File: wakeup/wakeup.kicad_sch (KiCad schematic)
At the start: 15 parts, among them J1 Conn_01x03_Female, U1 74HC00, U2 74HC393

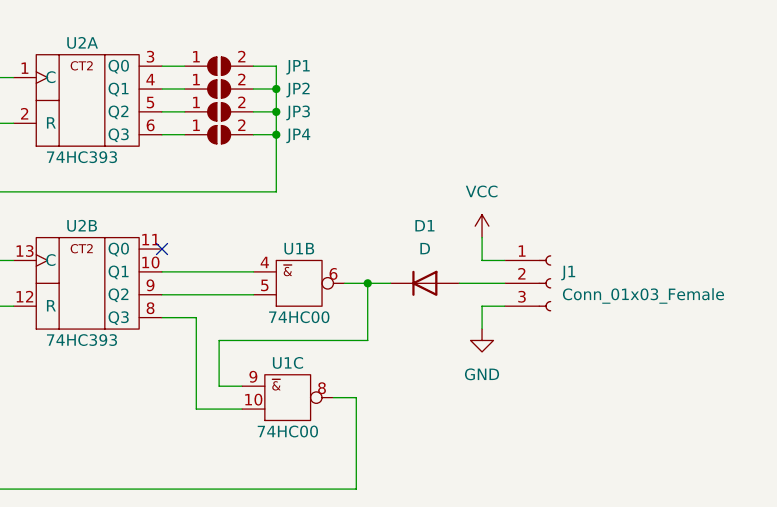
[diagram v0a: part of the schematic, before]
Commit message: non function changes
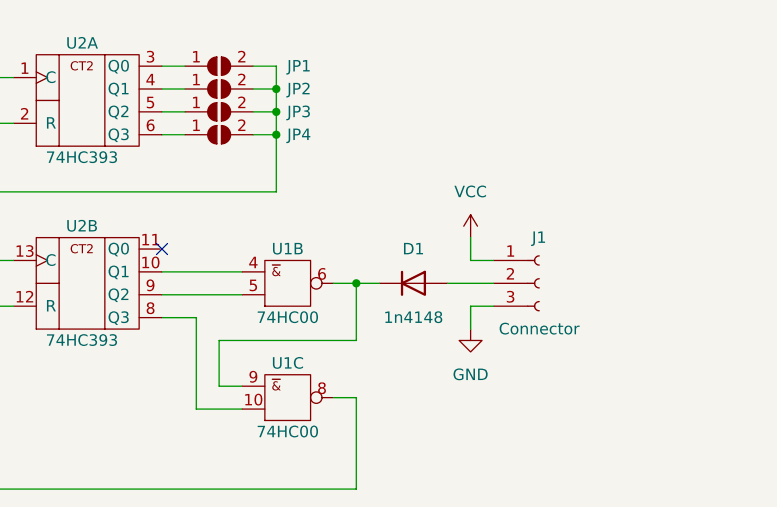
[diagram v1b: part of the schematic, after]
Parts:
- D1: value D -> 1n4148
- J1: value Conn_01x03_Female -> Connector
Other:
- moved on the sheet: D1, J1, U1B
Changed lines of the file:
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@@
   (junction (at 135.89 68.58) (diameter 0) (color 0 0 0 0)
   )
-  (junction (at 146.05 87.63) (diameter 0) (color 0 0 0 0)
+  (junction (at 144.78 87.63) (diameter 0) (color 0 0 0 0)
   )
   (junction (at 101.6 90.17) (diameter 0) (color 0 0 0 0)
@@
     (stroke (width 0) (type default) (color 0 0 0 0))
   )
-  (wire (pts (xy 158.75 92.71) (xy 158.75 90.17))
+  (wire (pts (xy 157.48 92.71) (xy 157.48 90.17))
     (stroke (width 0) (type default) (color 0 0 0 0))
   )
@@
     (stroke (width 0) (type default) (color 0 0 0 0))
   )
-  (wire (pts (xy 146.05 87.63) (xy 148.59 87.63))
+  (wire (pts (xy 144.78 87.63) (xy 147.32 87.63))
     (stroke (width 0) (type default) (color 0 0 0 0))
   )
@@
     (stroke (width 0) (type default) (color 0 0 0 0))
   )
-  (wire (pts (xy 158.75 82.55) (xy 158.75 85.09))
+  (wire (pts (xy 157.48 82.55) (xy 157.48 85.09))
     (stroke (width 0) (type default) (color 0 0 0 0))
   )
@@
     (stroke (width 0) (type default) (color 0 0 0 0))
   )
-  (wire (pts (xy 158.75 85.09) (xy 161.29 85.09))
+  (wire (pts (xy 157.48 85.09) (xy 160.02 85.09))
     (stroke (width 0) (type default) (color 0 0 0 0))
   )
@@
     (stroke (width 0) (type default) (color 0 0 0 0))
   )
-  (wire (pts (xy 146.05 93.98) (xy 129.54 93.98))
+  (wire (pts (xy 144.78 93.98) (xy 129.54 93.98))
     (stroke (width 0) (type default) (color 0 0 0 0))
   )
@@
     (stroke (width 0) (type default) (color 0 0 0 0))
   )
-  (wire (pts (xy 156.21 87.63) (xy 161.29 87.63))
+  (wire (pts (xy 154.94 87.63) (xy 160.02 87.63))
     (stroke (width 0) (type default) (color 0 0 0 0))
   )
@@
     (stroke (width 0) (type default) (color 0 0 0 0))
   )
-  (wire (pts (xy 146.05 87.63) (xy 146.05 93.98))
+  (wire (pts (xy 144.78 87.63) (xy 144.78 93.98))
     (stroke (width 0) (type default) (color 0 0 0 0))
   )
@@
     (stroke (width 0) (type default) (color 0 0 0 0))
   )
-  (wire (pts (xy 143.51 87.63) (xy 146.05 87.63))
+  (wire (pts (xy 142.24 87.63) (xy 144.78 87.63))
     (stroke (width 0) (type default) (color 0 0 0 0))
   )
@@
     (stroke (width 0) (type default) (color 0 0 0 0))
   )
-  (wire (pts (xy 158.75 90.17) (xy 161.29 90.17))
+  (wire (pts (xy 157.48 90.17) (xy 160.02 90.17))
     (stroke (width 0) (type default) (color 0 0 0 0))
   )
@@
     (stroke (width 0) (type default) (color 0 0 0 0))
   )
-  (wire (pts (xy 123.19 88.9) (xy 133.35 88.9))
+  (wire (pts (xy 123.19 88.9) (xy 132.08 88.9))
     (stroke (width 0) (type default) (color 0 0 0 0))
   )
@@
     (stroke (width 0) (type default) (color 0 0 0 0))
   )
-  (wire (pts (xy 123.19 86.36) (xy 133.35 86.36))
+  (wire (pts (xy 123.19 86.36) (xy 132.08 86.36))
     (stroke (width 0) (type default) (color 0 0 0 0))
   )
@@
     (pin "2")
   )
-  (symbol (lib_id "power:GND") (at 158.75 92.71 0) (unit 1)
-    (in_bom yes) (on_board yes) (fields_autoplaced)
-    (property "Reference" "#PWR07" (id 0) (at 158.75 99.06 0)
-      (effects (font (size 1.27 1.27)) hide)
-    )
-    (property "Value" "GND" (id 1) (at 158.75 97.79 0))
-    (property "Footprint" "" (id 2) (at 158.75 92.71 0)
-      (effects (font (size 1.27 1.27)) hide)
-    )
-    (property "Datasheet" "" (id 3) (at 158.75 92.71 0)
+  (symbol (lib_id "power:GND") (at 157.48 92.71 0) (unit 1)
+    (in_bom yes) (on_board yes) (fields_autoplaced)
+    (property "Reference" "#PWR07" (id 0) (at 157.48 99.06 0)
+      (effects (font (size 1.27 1.27)) hide)
+    )
+    (property "Value" "GND" (id 1) (at 157.48 97.79 0))
+    (property "Footprint" "" (id 2) (at 157.48 92.71 0)
+      (effects (font (size 1.27 1.27)) hide)
+    )
+    (property "Datasheet" "" (id 3) (at 157.48 92.71 0)
       (effects (font (size 1.27 1.27)) hide)
     )
@@
     (pin "13")
   )
-  (symbol (lib_id "74IEC:74HC00") (at 138.43 87.63 0) (unit 2)
-    (in_bom yes) (on_board yes)
-    (property "Reference" "U1" (id 0) (at 138.43 83.82 0))
-    (property "Value" "74HC00" (id 1) (at 138.43 91.44 0))
-    (property "Footprint" "Package_SO:SO-14_3.9x8.65mm_P1.27mm" (id 2) (at 138.43 93.98 0)
-      (effects (font (size 1.27 1.27)) hide)
-    )
-    (property "Datasheet" "https://www.ti.com/lit/ds/symlink/sn7400.pdf" (id 3) (at 138.43 83.82 0)
+  (symbol (lib_id "74IEC:74HC00") (at 137.16 87.63 0) (unit 2)
+    (in_bom yes) (on_board yes)
+    (property "Reference" "U1" (id 0) (at 137.16 83.82 0))
+    (property "Value" "74HC00" (id 1) (at 137.16 91.44 0))
+    (property "Footprint" "Package_SO:SO-14_3.9x8.65mm_P1.27mm" (id 2) (at 137.16 93.98 0)
+      (effects (font (size 1.27 1.27)) hide)
+    )
+    (property "Datasheet" "https://www.ti.com/lit/ds/symlink/sn7400.pdf" (id 3) (at 137.16 83.82 0)
       (effects (font (size 1.27 1.27)) hide)
     )
@@
     (pin "2")
   )
-  (symbol (lib_id "Device:D") (at 152.4 87.63 0) (unit 1)
-    (in_bom yes) (on_board yes) (fields_autoplaced)
-    (property "Reference" "D1" (id 0) (at 152.4 81.28 0))
-    (property "Value" "D" (id 1) (at 152.4 83.82 0))
-    (property "Footprint" "" (id 2) (at 152.4 87.63 0)
-      (effects (font (size 1.27 1.27)) hide)
-    )
-    (property "Datasheet" "~" (id 3) (at 152.4 87.63 0)
+  (symbol (lib_id "Device:D") (at 151.13 87.63 0) (unit 1)
+    (in_bom yes) (on_board yes)
+    (property "Reference" "D1" (id 0) (at 151.13 83.82 0))
+    (property "Value" "1n4148" (id 1) (at 151.13 91.44 0))
+    (property "Footprint" "" (id 2) (at 151.13 87.63 0)
+      (effects (font (size 1.27 1.27)) hide)
+    )
+    (property "Datasheet" "~" (id 3) (at 151.13 87.63 0)
       (effects (font (size 1.27 1.27)) hide)
     )
@@
     (pin "9")
   )
-  (symbol (lib_id "power:VCC") (at 158.75 82.55 0) (unit 1)
-    (in_bom yes) (on_board yes) (fields_autoplaced)
-    (property "Reference" "#PWR05" (id 0) (at 158.75 86.36 0)
-      (effects (font (size 1.27 1.27)) hide)
-    )
-    (property "Value" "VCC" (id 1) (at 158.75 77.47 0))
-    (property "Footprint" "" (id 2) (at 158.75 82.55 0)
-      (effects (font (size 1.27 1.27)) hide)
-    )
-    (property "Datasheet" "" (id 3) (at 158.75 82.55 0)
+  (symbol (lib_id "power:VCC") (at 157.48 82.55 0) (unit 1)
+    (in_bom yes) (on_board yes) (fields_autoplaced)
+    (property "Reference" "#PWR05" (id 0) (at 157.48 86.36 0)
+      (effects (font (size 1.27 1.27)) hide)
+    )
+    (property "Value" "VCC" (id 1) (at 157.48 77.47 0))
+    (property "Footprint" "" (id 2) (at 157.48 82.55 0)
+      (effects (font (size 1.27 1.27)) hide)
+    )
+    (property "Datasheet" "" (id 3) (at 157.48 82.55 0)
       (effects (font (size 1.27 1.27)) hide)
     )
@@
     (pin "13")
   )
-  (symbol (lib_id "Connector:Conn_01x03_Female") (at 166.37 87.63 0) (unit 1)
-    (in_bom yes) (on_board yes) (fields_autoplaced)
-    (property "Reference" "J1" (id 0) (at 167.64 86.3599 0)
-      (effects (font (size 1.27 1.27)) (justify left))
-    )
-    (property "Value" "Conn_01x03_Female" (id 1) (at 167.64 88.8999 0)
-      (effects (font (size 1.27 1.27)) (justify left))
-    )
-    (property "Footprint" "Connector_PinSocket_2.54mm:PinSocket_1x03_P2.54mm_Vertical" (id 2) (at 166.37 87.63 0)
-      (effects (font (size 1.27 1.27)) hide)
-    )
-    (property "Datasheet" "~" (id 3) (at 166.37 87.63 0)
+  (symbol (lib_id "Connector:Conn_01x03_Female") (at 165.1 87.63 0) (unit 1)
+    (in_bom yes) (on_board yes)
+    (property "Reference" "J1" (id 0) (at 165.1 82.55 0))
+    (property "Value" "Connector" (id 1) (at 165.1 92.71 0))
+    (property "Footprint" "Connector_PinSocket_2.54mm:PinSocket_1x03_P2.54mm_Vertical" (id 2) (at 165.1 87.63 0)
+      (effects (font (size 1.27 1.27)) hide)
+    )
+    (property "Datasheet" "~" (id 3) (at 165.1 87.63 0)
       (effects (font (size 1.27 1.27)) hide)
     )
@@
     )
     (path "/73e9b2dc-e516-489c-bad5-4d0f9f05c72b"
-      (reference "D1") (unit 1) (value "D") (footprint "")
+      (reference "D1") (unit 1) (value "1n4148") (footprint "")
     )
     (path "/c0ac4adc-1766-46e3-9139-a9cacdb1fe63"
-      (reference "J1") (unit 1) (value "Conn_01x03_Female") (footprint "Connector_PinSocket_2.54mm:PinSocket_1x03_P2.54mm_Vertical")
+      (reference "J1") (unit 1) (value "Connector") (footprint "Connector_PinSocket_2.54mm:PinSocket_1x03_P2.54mm_Vertical")
     )
     (path "/a71539b7-6be1-48ce-a90f-d231122870e8"
